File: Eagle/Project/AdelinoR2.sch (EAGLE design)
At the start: 70 parts, among them J1 DC-044-A, J2 YELLOW-8P-2.54, J3 YELLOW-6P-2.54, J4 YELLOW-8P-2.54, J5 YELLOW-8P-2.54, J6 4P-2.0, J7 YELLOW-2X3P-2.54, J8 4P-2.0, Q1 NCE3407A, Q2 CJ2305, SW1 TS-1101F, U1 MP1496DJ-SOT23-8, U2 CJT1117-3.3-SOT223, U3 ESP-12F / OPL: 317060163 / SM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, U4 ATMEGA32U4-MUR-QFN44, U5 74VHC125MTCX-TSSOP14, U6 ATMEGA32U4-TQFP44, X1 306010049_XTAL_16MHZ-3225_4P

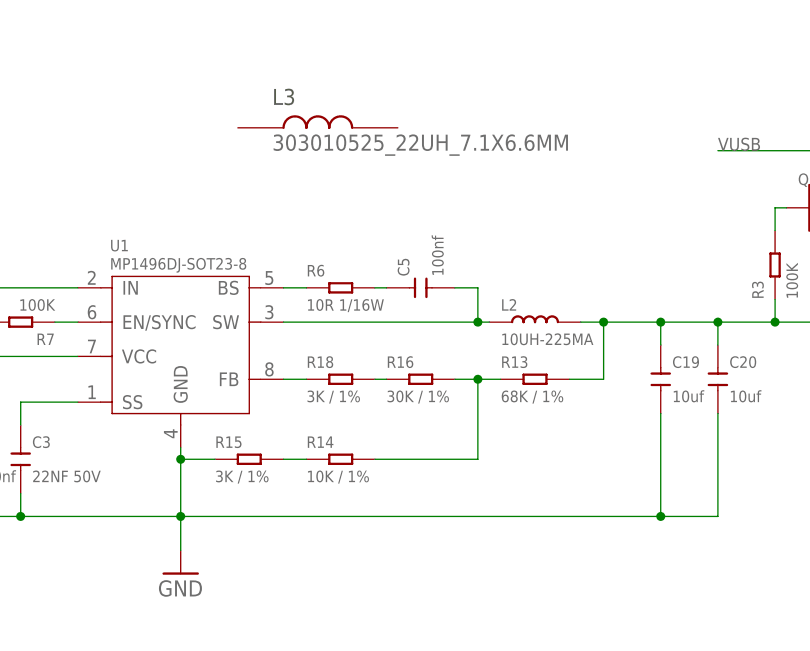
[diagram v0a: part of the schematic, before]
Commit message: Power supply routing wip.
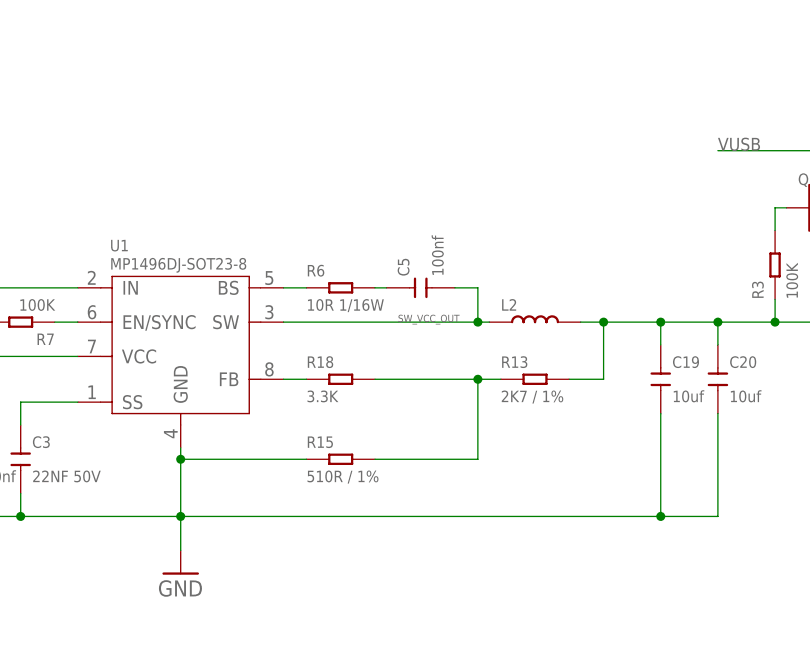
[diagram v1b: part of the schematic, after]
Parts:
- removed L3: 303010525_22UH_7.1X6.6MM, Seeed-OPL-2017-01-Inductor-Akita:303010525_22UH_7.1X6.6MM
- removed R14: 10K / 1%, Seeed-Resistor:SMD-RES-10K-1%-1/10W(0603)
- removed R16: 30K / 1%, Seeed-Resistor:SMD-RES-30K-1%-1/10W(0603)
- L2: device Seeed-Inductor:SMD-INDUCTOR-10UH-225MA-10%(0806) -> Seeed-Inductor:SMD-INDUCTOR-10UH-20%-2.35A(2P-5X5X4MM)
- R13: value 68K / 1% -> 2K7 / 1%; device Seeed-Resistor:SMD-RES-68K-1%-1/10W(0603) -> Seeed-Resistor:SMD-RES-2.7K-1%-1/10W(0603); R (none) -> 2K7 / 1%
- R15: device Seeed-Resistor:SMD-RES-3K-1%-1/10W(0603) -> Seeed-Resistor:SMD-RES-510R-1%-1/10W(0603); R (none) -> 510R / 1%
- R18: value 3K / 1% -> 3.3K; device Seeed-Resistor:SMD-RES-3K-1%-1/10W(0603) -> Seeed-Resistor:SMD-RES-3.3K-5%-1/16W(0402)
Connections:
- net N$10 renamed SW_VCC_IN
- net N$12 renamed SW_VCAP
- net N$14 renamed SW_BS
- net N$19 renamed SW_VCC_OUT
- net N$20 renamed SW_EN
- net N$24 renamed SW_FB
- net N$4 renamed SW_SS
- removed net N$21: R16.1, R18.2
- removed net N$22: R14.1, R15.2
- net N$23: now also R15.2, R18.2; no longer R14.2, R16.2
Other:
- moved on the sheet: R15
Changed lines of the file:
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@@
 <setting verticaltext="up"/>
 </settings>
-<grid distance="0.05" unitdist="inch" unit="inch" style="lines" multiple="1" display="no" altdistance="0.01" altunitdist="inch" altunit="inch"/>
+<grid distance="0.1" unitdist="inch" unit="inch" style="lines" multiple="1" display="no" altdistance="0.01" altunitdist="inch" altunit="inch"/>
 <layers>
 <layer number="1" name="Top" color="4" fill="1" visible="no" active="no"/>
@@
 <classes>
 <class number="0" name="default" width="0.254" drill="0.6096">
-<clearance class="0" value="0.254"/>
+<clearance class="0" value="0.2032"/>
 </class>
 </classes>
@@
 <part name="R6" library="Seeed-Resistor" deviceset="SMD-RES-10R-1%-1/16W(0402)" device="" value="10R 1/16W"/>
 <part name="C5" library="Seeed-Capacitor" deviceset="CERAMIC-100NF-25V-10%-X7R(0402)" device="" value="100nf"/>
-<part name="L2" library="Seeed-Inductor" deviceset="SMD-INDUCTOR-10UH-225MA-10%(0806)" device="" value="10UH-225MA"/>
+<part name="L2" library="Seeed-Inductor" deviceset="SMD-INDUCTOR-10UH-20%-2.35A(2P-5X5X4MM)" device="" value="10UH-225MA"/>
 <part name="R7" library="Seeed-Resistor" deviceset="SMD-RES-100K-1%-1/16W(0402)" device="" value="100K"/>
-<part name="R13" library="Seeed-Resistor" deviceset="SMD-RES-68K-1%-1/10W(0603)" device="" value="68K / 1%"/>
-<part name="R14" library="Seeed-Resistor" deviceset="SMD-RES-10K-1%-1/10W(0603)" device="" value="10K / 1%"/>
+<part name="R13" library="Seeed-Resistor" deviceset="SMD-RES-2.7K-1%-1/10W(0603)" device="" value="2K7 / 1%">
+<attribute name="R" value="2K7 / 1%"/>
+</part>
 <part name="GND15" library="supply1" library_urn="urn:adsk.eagle:library:371" deviceset="GND" device=""/>
-<part name="R16" library="Seeed-Resistor" deviceset="SMD-RES-30K-1%-1/10W(0603)" device="" value="30K / 1%"/>
 <part name="C19" library="Seeed-Capacitor" deviceset="CERAMIC-10UF-25V-10%-X5R(0805)" device="" value="10uf"/>
 <part name="C20" library="Seeed-Capacitor" deviceset="CERAMIC-10UF-25V-10%-X5R(0805)" device="" value="10uf"/>
-<part name="R15" library="Seeed-Resistor" deviceset="SMD-RES-3K-1%-1/10W(0603)" device="" value="3K / 1%"/>
-<part name="R18" library="Seeed-Resistor" deviceset="SMD-RES-3K-1%-1/10W(0603)" device="" value="3K / 1%"/>
+<part name="R15" library="Seeed-Resistor" deviceset="SMD-RES-510R-1%-1/10W(0603)" device="" value="3K / 1%">
+<attribute name="R" value="510R / 1%"/>
+</part>
+<part name="R18" library="Seeed-Resistor" deviceset="SMD-RES-3.3K-5%-1/16W(0402)" device="" value="3.3K"/>
 <part name="U6" library="Seeed-IC" deviceset="MCU-ATMEGA32U4-AU(TQFP44)" device="" value="ATMEGA32U4-TQFP44">
 <attribute name="DESC" value="SOCKET B - TQFP44"/>
 </part>
-<part name="L3" library="Seeed-OPL-2017-01-Inductor-Akita" deviceset="303010525_22UH_7.1X6.6MM" device=""/>
 <part name="GND2" library="supply1" library_urn="urn:adsk.eagle:library:371" deviceset="GND" device=""/>
 <part name="P+8" library="supply1" library_urn="urn:adsk.eagle:library:371" deviceset="+5V" device=""/>
@@
 <attribute name="VALUE" x="-123.19" y="148.59" size="1.27" layer="96" ratio="10" rot="R90"/>
 </instance>
-<instance part="L2" gate="L" x="-113.03" y="143.51" smashed="yes">
+<instance part="L2" gate="G$1" x="-113.03" y="143.51" smashed="yes">
 <attribute name="NAME" x="-116.84" y="144.78" size="1.27" layer="95" ratio="10"/>
-<attribute name="VALUE" x="-116.84" y="140.97" size="1.27" layer="96" ratio="10"/>
 </instance>
 <instance part="R7" gate="G$1" x="-170.18" y="143.51" smashed="yes" rot="R180">
@@
 <instance part="R13" gate="G$1" x="-113.03" y="137.16" smashed="yes">
 <attribute name="NAME" x="-116.84" y="138.43" size="1.27" layer="95" ratio="10"/>
-<attribute name="VALUE" x="-116.84" y="134.62" size="1.27" layer="96" ratio="10"/>
-</instance>
-<instance part="R14" gate="G$1" x="-134.62" y="128.27" smashed="yes">
-<attribute name="NAME" x="-138.43" y="129.54" size="1.27" layer="95" ratio="10"/>
-<attribute name="VALUE" x="-138.43" y="125.73" size="1.27" layer="96" ratio="10"/>
+<attribute name="R" x="-116.84" y="134.62" size="1.27" layer="96"/>
 </instance>
 <instance part="GND15" gate="1" x="-152.4" y="115.57" smashed="yes">
 <attribute name="VALUE" x="-154.94" y="113.03" size="1.778" layer="96"/>
-</instance>
-<instance part="R16" gate="G$1" x="-125.73" y="137.16" smashed="yes">
-<attribute name="NAME" x="-129.54" y="138.43" size="1.27" layer="95" ratio="10"/>
-<attribute name="VALUE" x="-129.54" y="134.62" size="1.27" layer="96" ratio="10"/>
 </instance>
 <instance part="C19" gate="G$1" x="-99.06" y="137.16" smashed="yes" rot="R90">
@@
 <attribute name="VALUE" x="-91.44" y="134.62" size="1.27" layer="96" ratio="10"/>
 </instance>
-<instance part="R15" gate="G$1" x="-144.78" y="128.27" smashed="yes">
-<attribute name="NAME" x="-148.59" y="129.54" size="1.27" layer="95" ratio="10"/>
-<attribute name="VALUE" x="-148.59" y="125.73" size="1.27" layer="96" ratio="10"/>
+<instance part="R15" gate="G$1" x="-134.62" y="128.27" smashed="yes">
+<attribute name="NAME" x="-138.43" y="129.54" size="1.27" layer="95" ratio="10"/>
+<attribute name="R" x="-138.43" y="125.73" size="1.27" layer="96"/>
 </instance>
 <instance part="R18" gate="G$1" x="-134.62" y="137.16" smashed="yes">
@@
 <attribute name="VALUE" x="201.93" y="135.89" size="1.778" layer="96"/>
 <attribute name="DESC" x="201.93" y="133.35" size="1.778" layer="96"/>
-</instance>
-<instance part="L3" gate="G$1" x="-137.16" y="165.1" smashed="yes">
-<attribute name="NAME" x="-142.24" y="167.64" size="1.778" layer="97"/>
-<attribute name="VALUE" x="-142.24" y="162.56" size="1.778" layer="96"/>
 </instance>
 <instance part="GND2" gate="1" x="163.83" y="50.8" smashed="yes">
@@
 <junction x="-99.06" y="121.92"/>
 <pinref part="R15" gate="G$1" pin="1"/>
-<wire x1="-148.59" y1="128.27" x2="-152.4" y2="128.27" width="0.1524" layer="91"/>
+<wire x1="-138.43" y1="128.27" x2="-152.4" y2="128.27" width="0.1524" layer="91"/>
 <junction x="-152.4" y="128.27"/>
 <pinref part="C3" gate="G$1" pin="1"/>
@@
 <wire x1="-92.71" y1="143.51" x2="-86.36" y2="143.51" width="0.1524" layer="91"/>
 <junction x="-86.36" y="143.51"/>
-<pinref part="L2" gate="L" pin="2"/>
+<pinref part="L2" gate="G$1" pin="2"/>
 <wire x1="-107.95" y1="143.51" x2="-105.41" y2="143.51" width="0.1524" layer="91"/>
 <wire x1="-105.41" y1="143.51" x2="-99.06" y2="143.51" width="0.1524" layer="91"/>
@@
 </segment>
 </net>
-<net name="N$10" class="0">
+<net name="SW_VCC_IN" class="0">
 <segment>
 <pinref part="Q1" gate="G$1" pin="S"/>
@@
 </segment>
 </net>
-<net name="N$12" class="0">
+<net name="SW_VCAP" class="0">
 <segment>
 <pinref part="U1" gate="G$1" pin="VCC"/>
@@
 </segment>
 </net>
-<net name="N$14" class="0">
+<net name="SW_BS" class="0">
 <segment>
 <pinref part="U1" gate="G$1" pin="BS"/>
@@
 </segment>
 </net>
-<net name="N$19" class="0">
+<net name="SW_VCC_OUT" class="0">
 <segment>
 <pinref part="U1" gate="G$1" pin="SW"/>
-<pinref part="L2" gate="L" pin="1"/>
+<pinref part="L2" gate="G$1" pin="1"/>
 <wire x1="-140.97" y1="143.51" x2="-119.38" y2="143.51" width="0.1524" layer="91"/>
 <pinref part="C5" gate="G$1" pin="1"/>
@@
 <wire x1="-119.38" y1="147.32" x2="-119.38" y2="143.51" width="0.1524" layer="91"/>
 <junction x="-119.38" y="143.51"/>
-</segment>
-</net>
-<net name="N$20" class="0">
+<label x="-128.27" y="143.51" size="0.8128" layer="95"/>
+</segment>
+</net>
+<net name="SW_EN" class="0">
 <segment>
 <pinref part="U1" gate="G$1" pin="EN/SYNC"/>
@@
 <net name="N$23" class="0">
 <segment>
-<pinref part="R16" gate="G$1" pin="2"/>
 <pinref part="R13" gate="G$1" pin="1"/>
-<wire x1="-116.84" y1="137.16" x2="-119.38" y2="137.16" width="0.1524" layer="91"/>
-<pinref part="R14" gate="G$1" pin="2"/>
-<wire x1="-119.38" y1="137.16" x2="-121.92" y2="137.16" width="0.1524" layer="91"/>
+<pinref part="R18" gate="G$1" pin="2"/>
+<wire x1="-130.81" y1="137.16" x2="-119.38" y2="137.16" width="0.1524" layer="91"/>
+<pinref part="R15" gate="G$1" pin="2"/>
+<wire x1="-119.38" y1="137.16" x2="-116.84" y2="137.16" width="0.1524" layer="91"/>
 <wire x1="-130.81" y1="128.27" x2="-119.38" y2="128.27" width="0.1524" layer="91"/>
 <wire x1="-119.38" y1="128.27" x2="-119.38" y2="137.16" width="0.1524" layer="91"/>
@@
 </segment>
 </net>
-<net name="N$22" class="0">
-<segment>
-<pinref part="R14" gate="G$1" pin="1"/>
-<pinref part="R15" gate="G$1" pin="2"/>
-<wire x1="-138.43" y1="128.27" x2="-140.97" y2="128.27" width="0.1524" layer="91"/>
-</segment>
-</net>
-<net name="N$4" class="0">
+<net name="SW_SS" class="0">
 <segment>
 <pinref part="C3" gate="G$1" pin="2"/>
@@
 </segment>
 </net>
-<net name="N$21" class="0">
-<segment>
-<pinref part="R16" gate="G$1" pin="1"/>
-<pinref part="R18" gate="G$1" pin="2"/>
-<wire x1="-129.54" y1="137.16" x2="-130.81" y2="137.16" width="0.1524" layer="91"/>
-</segment>
-</net>
-<net name="N$24" class="0">
+<net name="SW_FB" class="0">
 <segment>
 <pinref part="R18" gate="G$1" pin="1"/>
